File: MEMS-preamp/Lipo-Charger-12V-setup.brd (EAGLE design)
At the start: 14 x 15.7 mm, 10 parts, among them U2 MIC5225-3.3

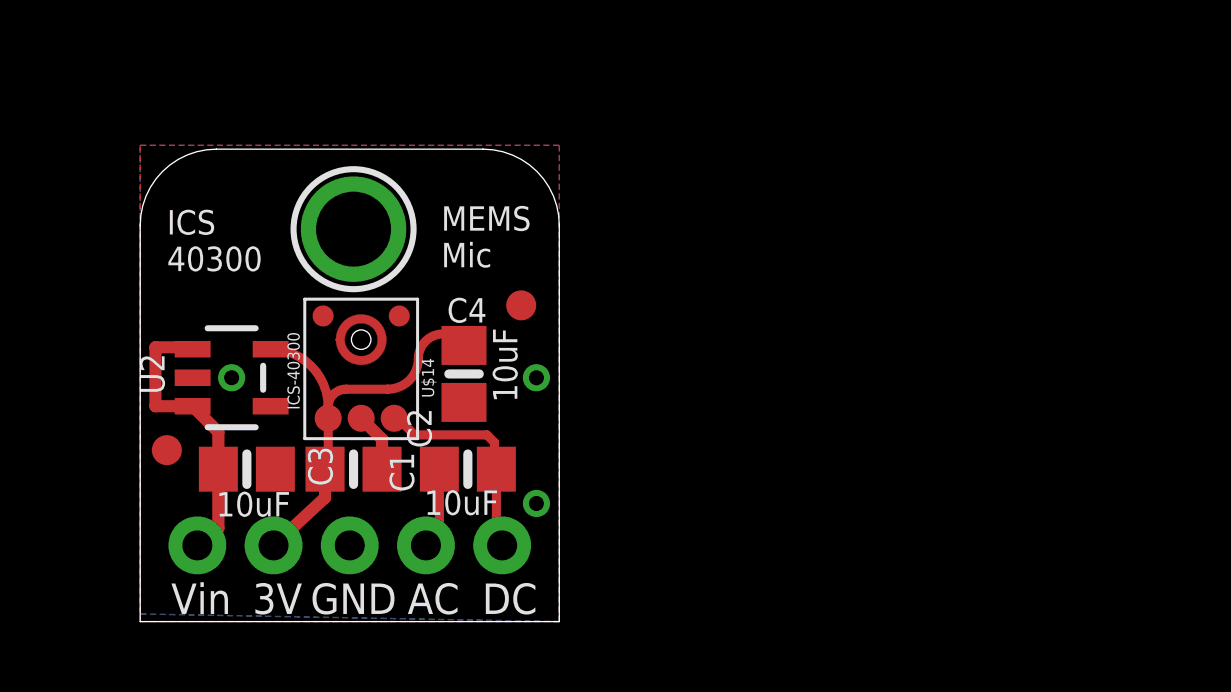
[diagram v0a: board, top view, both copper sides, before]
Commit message: many changes to chipchestra
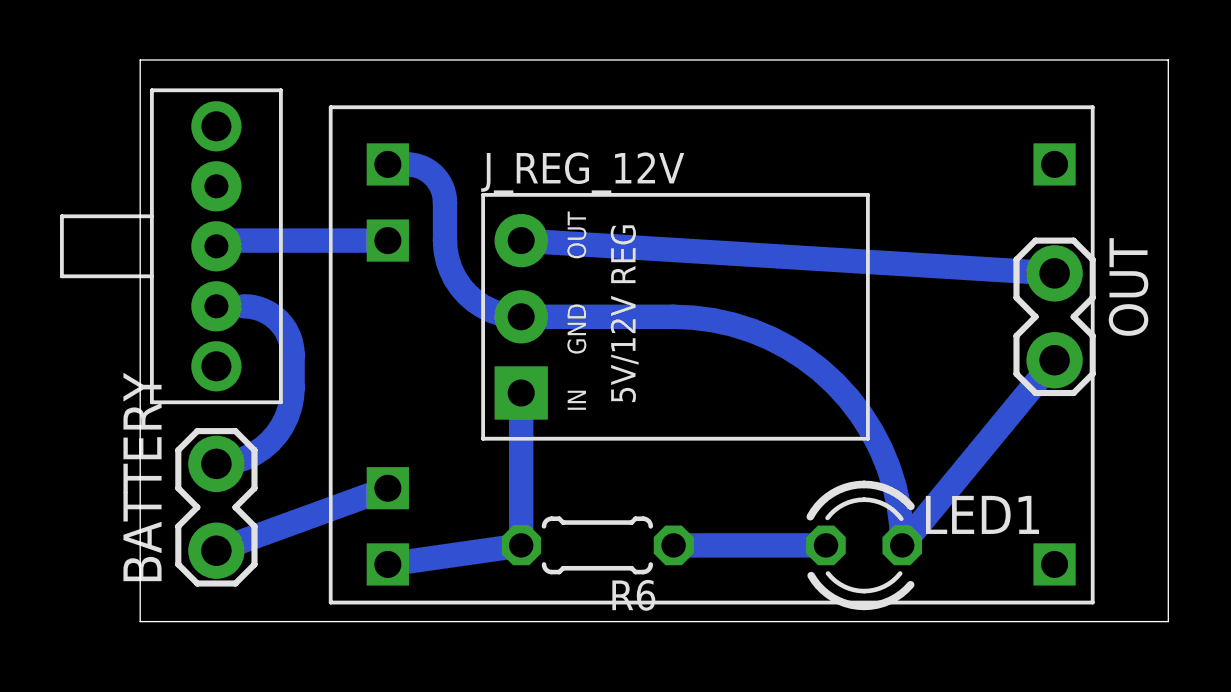
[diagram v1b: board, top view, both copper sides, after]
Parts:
- removed C1, C3, C4: 10uF, microbuilder:0805-NO
- removed C2: 0.1uF, microbuilder:0805-NO
- removed FID1, FID2: FIDUCIAL"", microbuilder:FIDUCIAL_1MM
- removed JP1: (no value), microbuilder:1X05_ROUND_76
- removed U$12: MOUNTINGHOLE2.5, microbuilder:MOUNTINGHOLE_2.5_PLATED
- removed U$14: ICS-40300, CMU-ArtFab:ICS-40300
- removed U2: MIC5225-3.3, microbuilder:SOT23-5
- added BATTERY, OUT: (no value), CMU-ArtFab:1X02_LOCK
- added J_REG_12V: POLOLU_VOLTAGE_REGULATORS_3PIN, CMU-ArtFab:POLOLU_5V-12V_STEPUP_U3V12F5-U3V12F12
- added LED1: (no value), led:LED3MM
- added POWER: SPDT, CMU-ArtFab:SWITCH_SPDT-TE-CONNECT
- added R6: 390, CMU-ArtFab:0204/5
- added USB-LIPO-CHARGER: TP4056-MODULE, CMU-ArtFab:TP4056-LITHIUM-PROTECTED-MODULE
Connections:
- removed net N$2: C1.1, JP1.4
- removed net VDD: C2.1, C4.1, JP1.2, U$14.P$5-VDD, U2.5
- new net +12V: J_REG_12V.VOUT, OUT.1
- new net IN+: USB-LIPO-CHARGER.IN+
- new net IN-: USB-LIPO-CHARGER.IN-
- new net N$16: LED1.A, R6.1
- new net N$18: BATTERY.1, USB-LIPO-CHARGER.B+
- new net N$19: POWER.2, USB-LIPO-CHARGER.B-
- net GND: now also J_REG_12V.GND, LED1.K, OUT.2, USB-LIPO-CHARGER.OUT-; no longer C2.2, C3.2, C4.2, JP1.3, U$14.P$2-GND, U$14.P$3-GND, U$14.P$4-GND, U$14.P$6-GND, U2.2
- net N$1: now also BATTERY.2, POWER.3; no longer C1.2, JP1.5, U$14.P$1-OUT
- net VIN: now also J_REG_12V.VIN, R6.2, USB-LIPO-CHARGER.OUT+; no longer C3.1, JP1.1, U2.1, U2.3
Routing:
- net GND: track 1.99 -> 31.1 mm, vias 3 -> 0
- net +12V: track 0.00 -> 17.8 mm
- net VDD: track 14.2 -> 0.00 mm
- net N$18: track 0.00 -> 6.08 mm
- net N$19: track 0.00 -> 5.91 mm
- net N$16: track 0.00 -> 5.08 mm
- net N$2: track 2.77 -> 0.00 mm
- removed copper zone on layer 1, net GND
- removed copper zone on layer 16, net GND
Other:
- board size 14 x 15.7 mm -> 34.3 x 18.7 mm
- board text removed: "3V"
- board text removed: "AC"
- board text removed: "DC"
- board text removed: "GND"
- board text removed: "ICS 40300"
- board text removed: "MEMS Mic"
- board text removed: "Vin"
